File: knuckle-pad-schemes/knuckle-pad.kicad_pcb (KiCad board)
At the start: 2 copper layers, 128 x 115.3 mm, 57 parts, among them SW1 SW_Push, SW10 SW_Push, SW11 SW_Push, SW12 SW_Push, SW13 SW_Push, SW14 SW_Push, SW15 SW_Push, SW16 SW_Push, SW17 SW_Push, SW18 SW_Push, SW19 SW_Push, SW2 SW_Push, SW20 SW_Push, SW21 SW_Push, SW22 SW_Push, SW23 SW_Push, SW24 SW_Push, SW25 SW_Push, SW26 SW_Push, SW27 SW_Push, SW3 SW_Push, SW4 SW_Push, SW5 SW_Push, SW6 SW_Push, SW7 SW_Push, SW8 SW_Push, SW9 SW_Push, U1 ProMicro

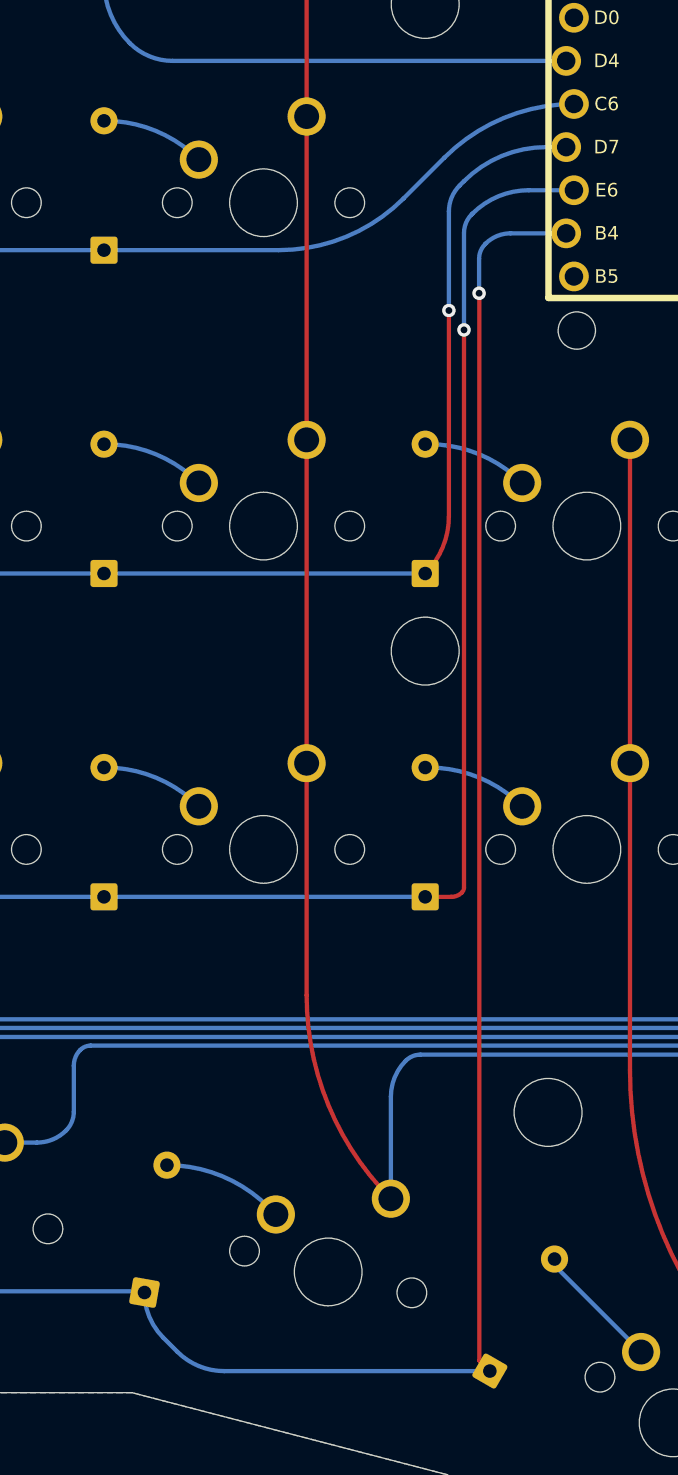
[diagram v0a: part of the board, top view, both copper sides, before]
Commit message: prelim version before trying to fit mcu cover and sw plate
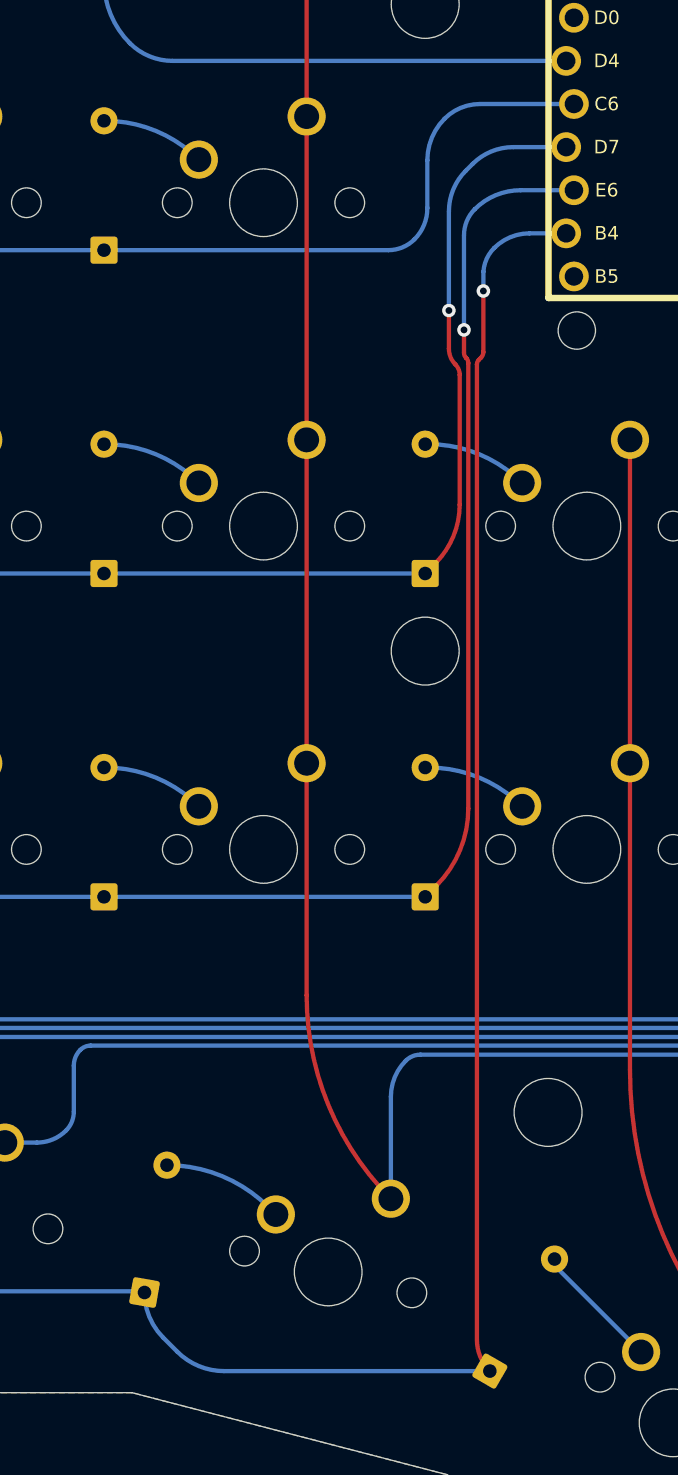
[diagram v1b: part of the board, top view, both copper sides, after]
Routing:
- net row1: track 91.4 -> 95.1 mm
- net row3: track 128.8 -> 126.8 mm
- net row4: track 163.6 -> 163.0 mm
